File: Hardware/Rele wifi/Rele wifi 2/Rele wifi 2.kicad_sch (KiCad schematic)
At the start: 15 parts, among them J1 Screw_Terminal_01x02, J2 Screw_Terminal_01x03, J3 Screw_Terminal_01x02, K1 G5LE-1, Q2 BC337, U5 PC817

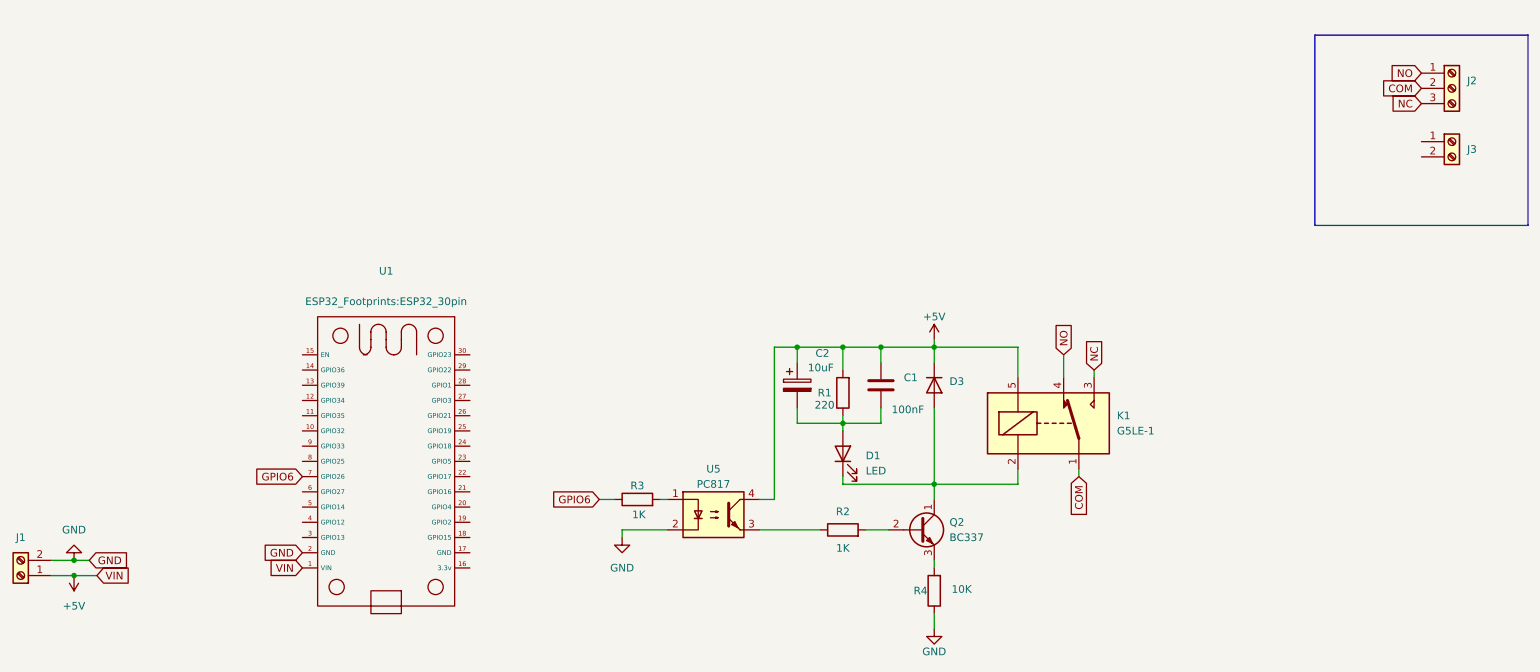
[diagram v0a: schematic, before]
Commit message: actu pcb
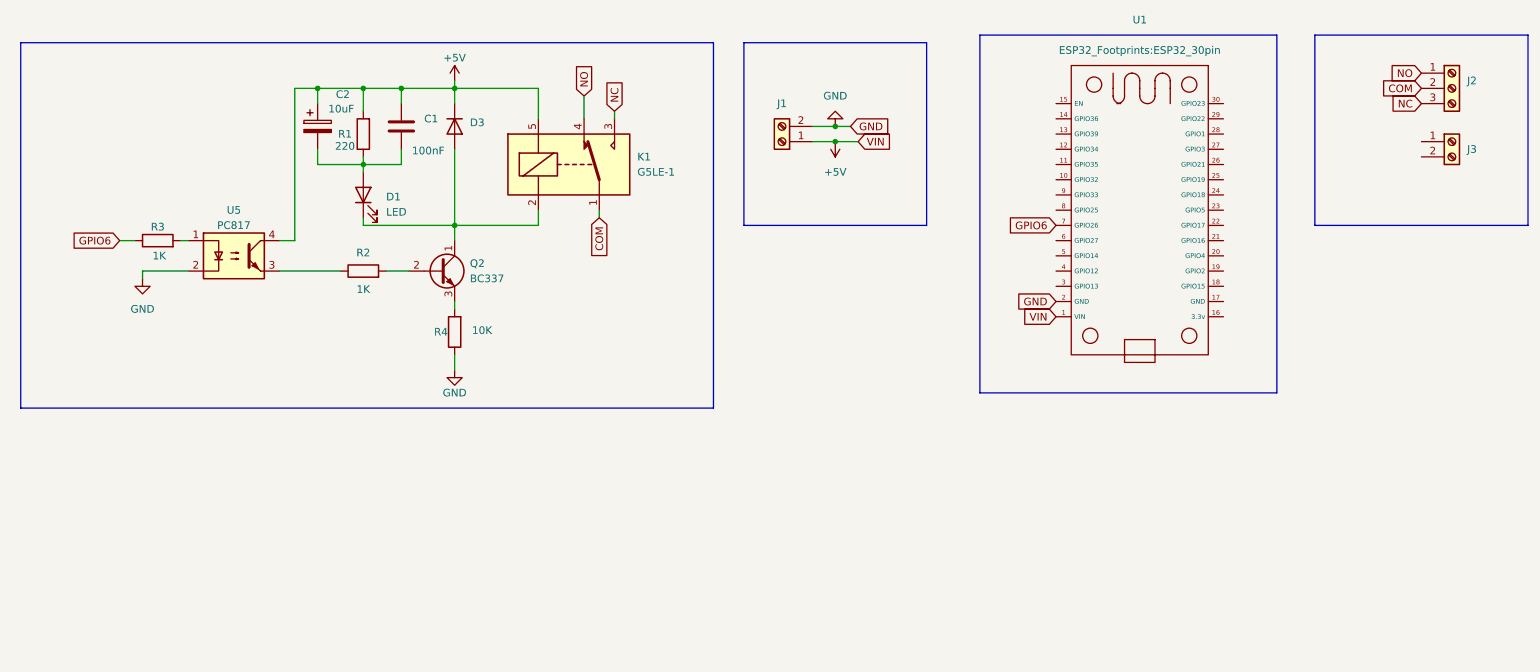
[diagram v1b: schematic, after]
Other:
- moved on the sheet: C1, C2, D1, D3, J1, K1, Q2, R1, R2, R3, R4, U1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

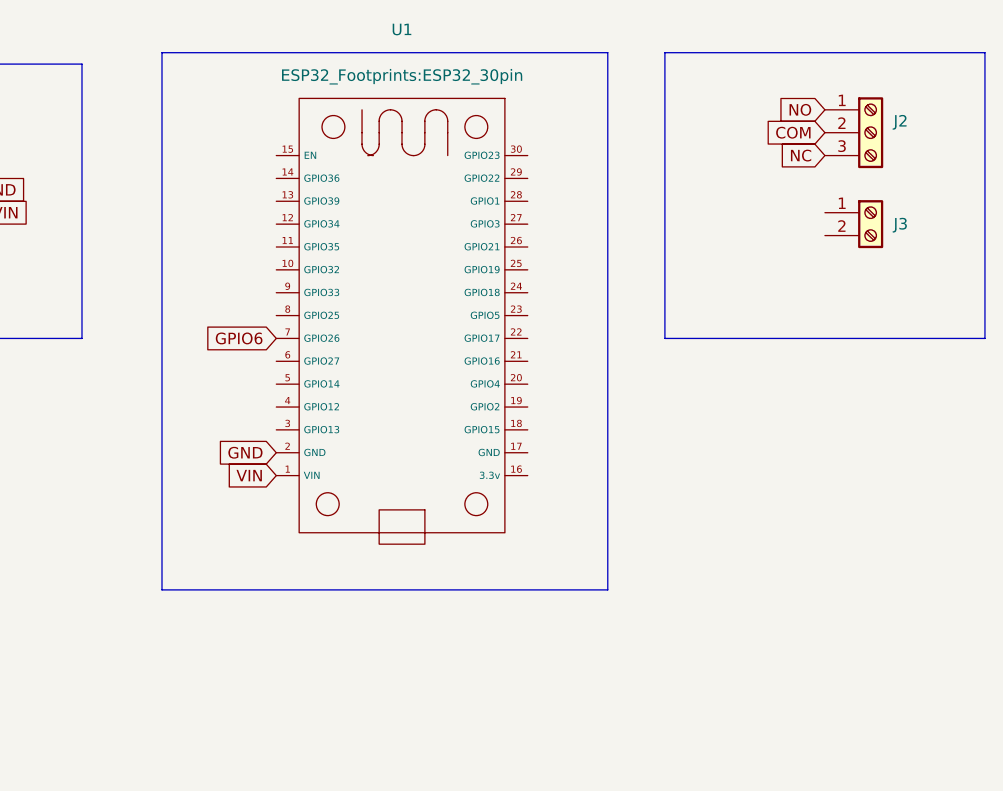
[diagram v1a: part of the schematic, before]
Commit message: act placa
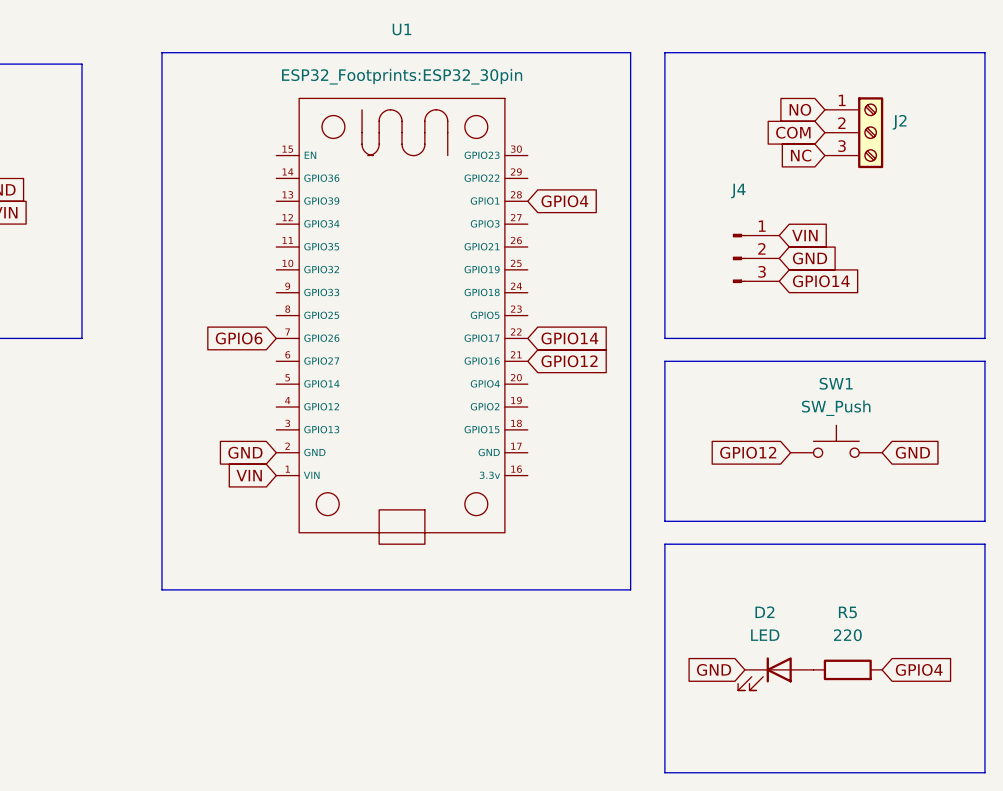
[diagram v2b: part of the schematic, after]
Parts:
- removed J3: Screw_Terminal_01x02, TerminalBlock:TerminalBlock_MaiXu_MX126-5.0-02P_1x02_P5.00mm, symbol Connector:Screw_Terminal_01x02
- added D2: LED, LED_THT:LED_D3.0mm_Clear, symbol Device:LED
- added J4: Conn_01x03_Pin, Connector_PinHeader_2.00mm:PinHeader_1x03_P2.00mm_Vertical, symbol Connector:Conn_01x03_Pin
- added R5: 220, Resistor_SMD:R_0805_2012Metric, symbol Device:R
- added SW1: SW_Push, Button_Switch_THT:SW_PUSH_1P1T_6x3.5mm_H5.0_APEM_MJTP1250, symbol Switch:SW_Push
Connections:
- net +5V: now also J4.1 (Pin_1)
- net GND: now also D2.1 (K), J4.2 (Pin_2), SW1.2
- net GPIO12: now reaches U1.21 (GPIO16)
- net GPIO12: now also SW1.1
- net GPIO14: now reaches U1.22 (GPIO17)
- net GPIO14: now also J4.3 (Pin_3)
- net GPIO4: now reaches U1.28 (GPIO1)
- net GPIO4: now also R5.2
- new net: D2.2 (A), R5.1
